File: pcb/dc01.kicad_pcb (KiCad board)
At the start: 4 copper layers, 76 x 84 mm, 103 parts, among them J1 USB_C_Receptacle_USB2.0, J10 MV132, J2 PROG/DEBUG, J3 Conn_01x06, J4 RJ12, J5 RJ12, J6 MV132, J7 MV132, J8 Conn_01x02, J9 MV132, K1 AZ850-5, K2 AZ850-5, Q1 2N7002, Q2 2N7002, SW1 SW_Push, SW2 SW_Push, SW3 MFP 113 D, U1 STM32F103C8Tx, U2 AMS1117-3.3, U3 PC817, U4 PC817, U5 PC817, U6 PC817, U7 74HC123, Y1 8 MHz

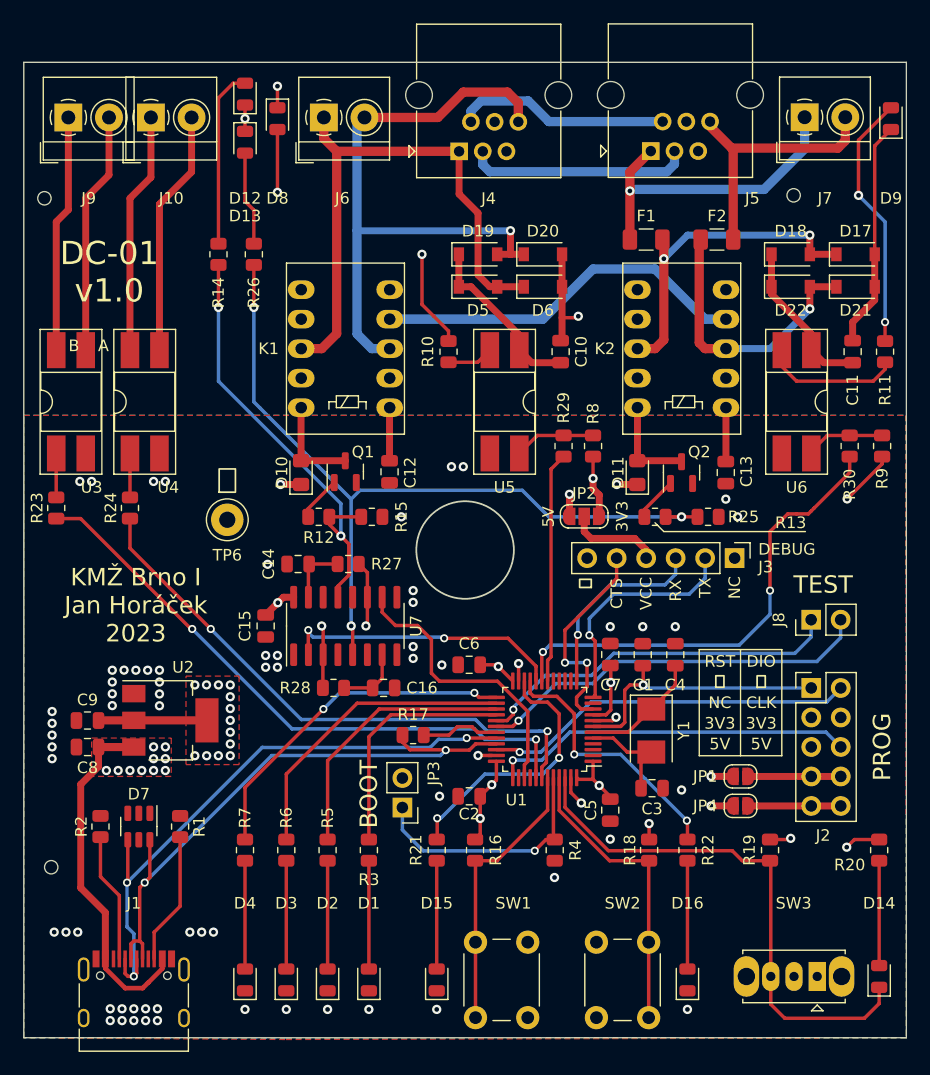
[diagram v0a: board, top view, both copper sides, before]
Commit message: Fix DRC errors.
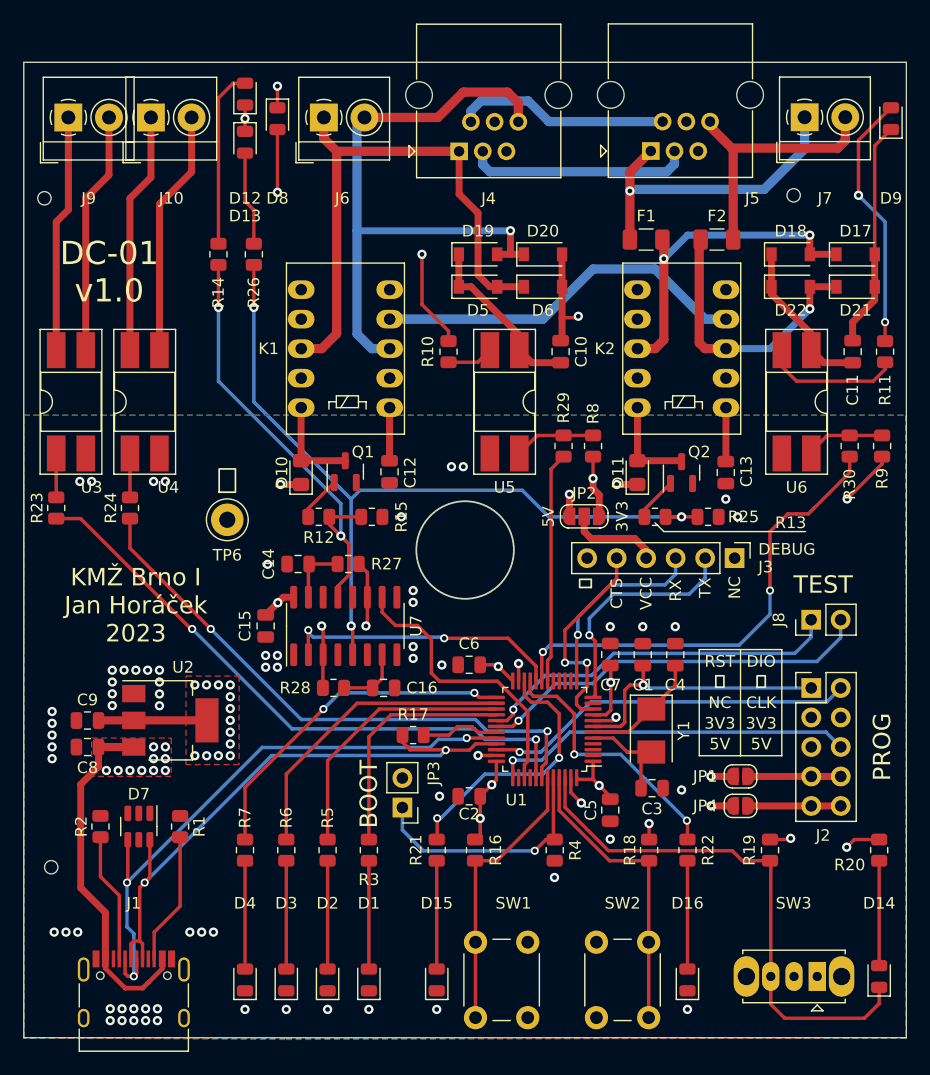
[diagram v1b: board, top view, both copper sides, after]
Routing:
- net Net-(J9-Pad2): track 21.5 -> 20.9 mm
- net Net-(J9-Pad1): track 21.2 -> 20.5 mm
- net Net-(J10-Pad1): track 21.5 -> 20.8 mm
- net Net-(J10-Pad2): track 21.9 -> 21.2 mm
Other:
- board text removed: "A"
- board text removed: "B"
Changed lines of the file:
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@@
     (effects (font (size 2 2) (thickness 0.15)))
-  )
-  (gr_text "A" (at 106.934 70.358) (layer "F.SilkS")
-    (effects (font (size 1 1) (thickness 0.15)))
   )
   (gr_text "VCC" (at 153.67 91.694 90) (layer "F.SilkS")
@@
   )
   (gr_text "3V3" (at 163.576 102.87) (layer "F.SilkS")
-    (effects (font (size 1 1) (thickness 0.15)))
-  )
-  (gr_text "B" (at 104.394 70.358) (layer "F.SilkS")
     (effects (font (size 1 1) (thickness 0.15)))
   )
@@
   (segment (start 119.126 50.8) (end 118.618 51.308) (width 0.3) (layer "In2.Cu") (net 2))
   (segment (start 118.618 51.308) (end 118.618 77.216) (width 0.3) (layer "In2.Cu") (net 2))
-  (segment (start 109.536 102.63) (end 109.55 102.616) (width 0.7) (layer "F.Cu") (net 3))
-  (segment (start 150.6235 109.156) (end 150.5575 109.156) (width 0.3) (layer "F.Cu") (net 3))
   (segment (start 149.098 102.14) (end 150.2075 102.14) (width 0.3) (layer "F.Cu") (net 3))
   (segment (start 150.5575 109.156) (end 149.62575 108.22425) (width 0.3) (layer "F.Cu") (net 3))
@@
   (segment (start 150.836 104.14) (end 152.042 105.346) (width 0.3) (layer "F.Cu") (net 4))
   (segment (start 149.098 104.14) (end 150.836 104.14) (width 0.3) (layer "F.Cu") (net 4))
-  (segment (start 154.178 105.4105) (end 154.1135 105.346) (width 0.3) (layer "F.Cu") (net 4))
   (segment (start 153.228 108.458) (end 153.228 106.2315) (width 0.3) (layer "F.Cu") (net 4))
   (segment (start 149.098 103.64) (end 152.1195 103.64) (width 0.3) (layer "F.Cu") (net 5))
@@
   (segment (start 102.87 59.69) (end 103.914 58.646) (width 0.6) (layer "F.Cu") (net 70))
   (segment (start 103.914 58.646) (end 103.914 50.7) (width 0.6) (layer "F.Cu") (net 70))
-  (segment (start 104.394 51.18) (end 103.914 50.7) (width 0.4) (layer "F.Cu") (net 70))
   (segment (start 105.41 57.658) (end 107.414 55.654) (width 0.6) (layer "F.Cu") (net 71))
   (segment (start 107.414 55.654) (end 107.414 50.7) (width 0.6) (layer "F.Cu") (net 71))
   (segment (start 105.41 70.739) (end 105.41 57.658) (width 0.6) (layer "F.Cu") (net 71))
-  (segment (start 106.934 51.18) (end 107.414 50.7) (width 0.4) (layer "F.Cu") (net 71))
   (segment (start 109.22 57.658) (end 111.026 55.852) (width 0.6) (layer "F.Cu") (net 72))
   (segment (start 109.22 70.739) (end 109.22 57.658) (width 0.6) (layer "F.Cu") (net 72))
   (segment (start 111.026 55.852) (end 111.026 50.7) (width 0.6) (layer "F.Cu") (net 72))
-  (segment (start 111.506 51.18) (end 111.026 50.7) (width 0.4) (layer "F.Cu") (net 72))
-  (segment (start 114.046 51.18) (end 114.526 50.7) (width 0.4) (layer "F.Cu") (net 73))
   (segment (start 111.76 58.166) (end 114.526 55.4) (width 0.6) (layer "F.Cu") (net 73))
   (segment (start 111.76 70.739) (end 111.76 58.166) (width 0.6) (layer "F.Cu") (net 73))
